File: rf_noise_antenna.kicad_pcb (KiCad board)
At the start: 2 copper layers, 65 x 56.5 mm, 41 parts, among them J1 Conn_Coaxial, J2 Conn_Coaxial, J3 Conn_01x03, J4 Raspberry_Pi_2_3, K1 MASWSS0115, K2 MASWSS0115, Q1 BC817, Q2 BC817, T1 MABA-009180-500MHz_1P_1S, U1 L7809

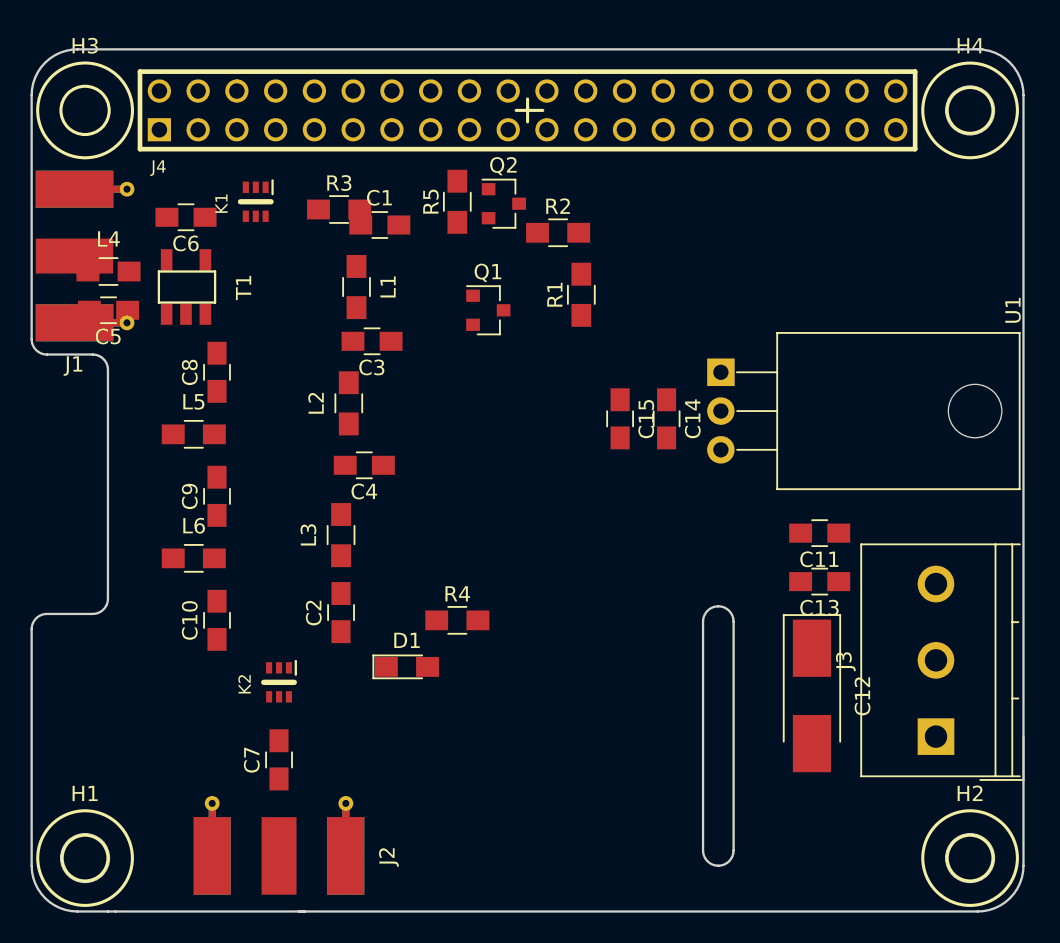
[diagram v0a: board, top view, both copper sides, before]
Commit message: Starting with PCB Layout
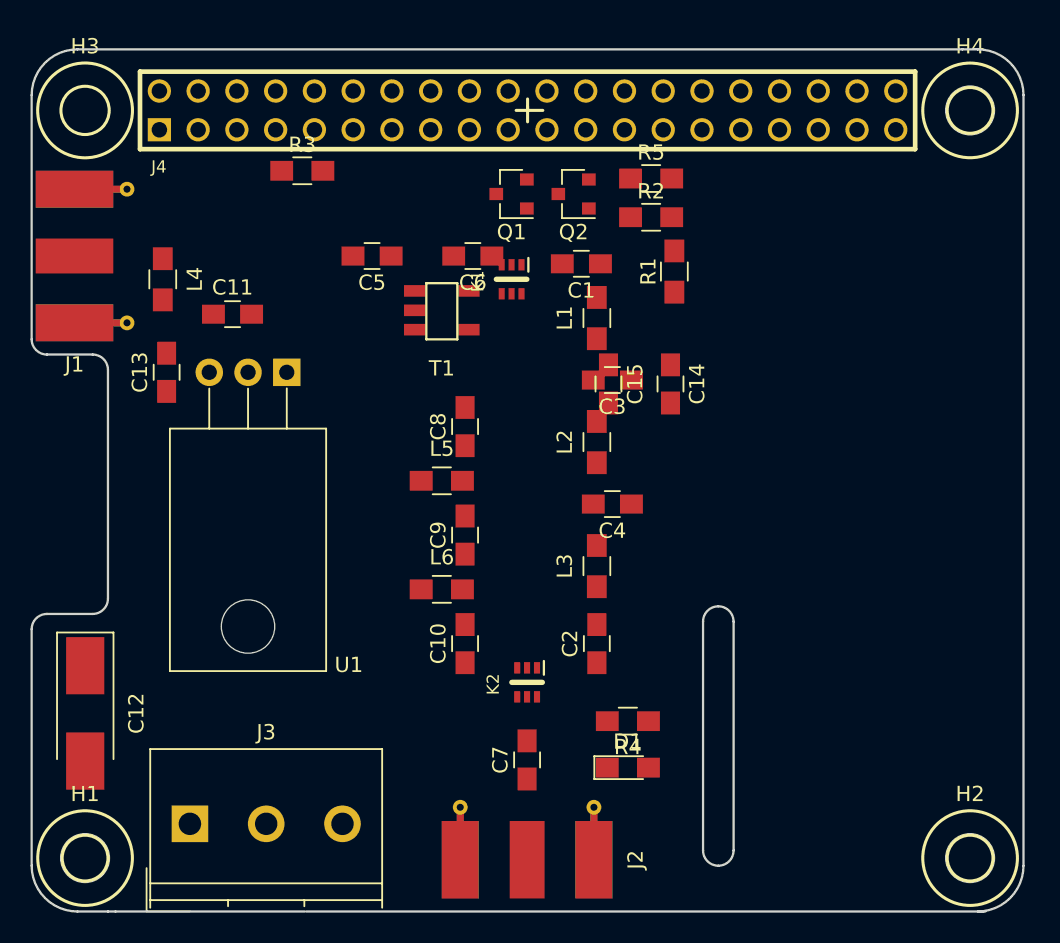
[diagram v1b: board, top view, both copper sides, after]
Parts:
- moved J3 49.2 mm to (39.4, 71.8), turned to 0 degrees
- moved C12 47.6 mm to (32.5, 64.5)
- moved C13 44.9 mm to (37.8, 42.2), turned to 90 degrees
- moved C11 41.1 mm to (42.2, 38.4), turned to 0 degrees
- moved U1 28.4 mm to (45.7, 42.2), turned to 180 degrees
- moved C6 19.0 mm to (57.9, 34.5)
- moved C5 17.6 mm to (51.3, 34.5)
- moved K1 17.5 mm to (60.5, 36.1)
- moved C2 16.9 mm to (66.0, 59.9)
- moved L3 16.9 mm to (66.0, 54.9)
- moved T1 16.8 mm to (55.9, 38.1), turned to 0 degrees
- moved C8 16.6 mm to (57.4, 45.7)
- moved L5 16.5 mm to (55.9, 49.3)
- moved L2 16.5 mm to (66.0, 46.7)
- moved C4 16.5 mm to (67.1, 50.8)
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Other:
- outline, holes or cut-outs redrawn
